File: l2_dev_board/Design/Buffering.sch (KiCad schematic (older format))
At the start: 32 parts, among them U202 NC7WZ07, U203 NC7WZ07, U204 NC7WZ07, U205 NC7WZ07, U302 NC7WZ17, U303 NC7WZ17, U304 NC7WZ17, U305 NC7WZ17, U306 NC7WZ17, U307 NC7WZ17, U310 NC7WZ17, U311 NC7WZ17

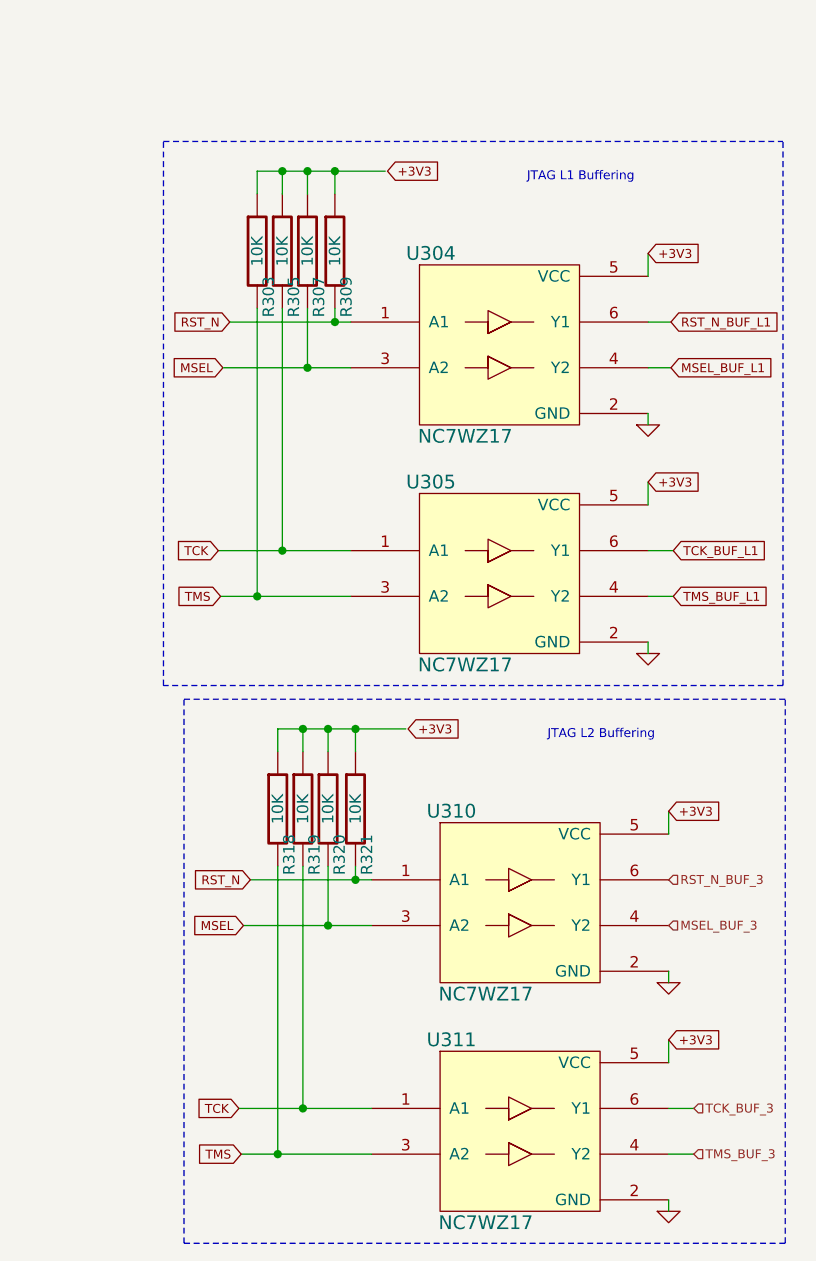
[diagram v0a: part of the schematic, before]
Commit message: missing header connector for 2 L2s. Find space!
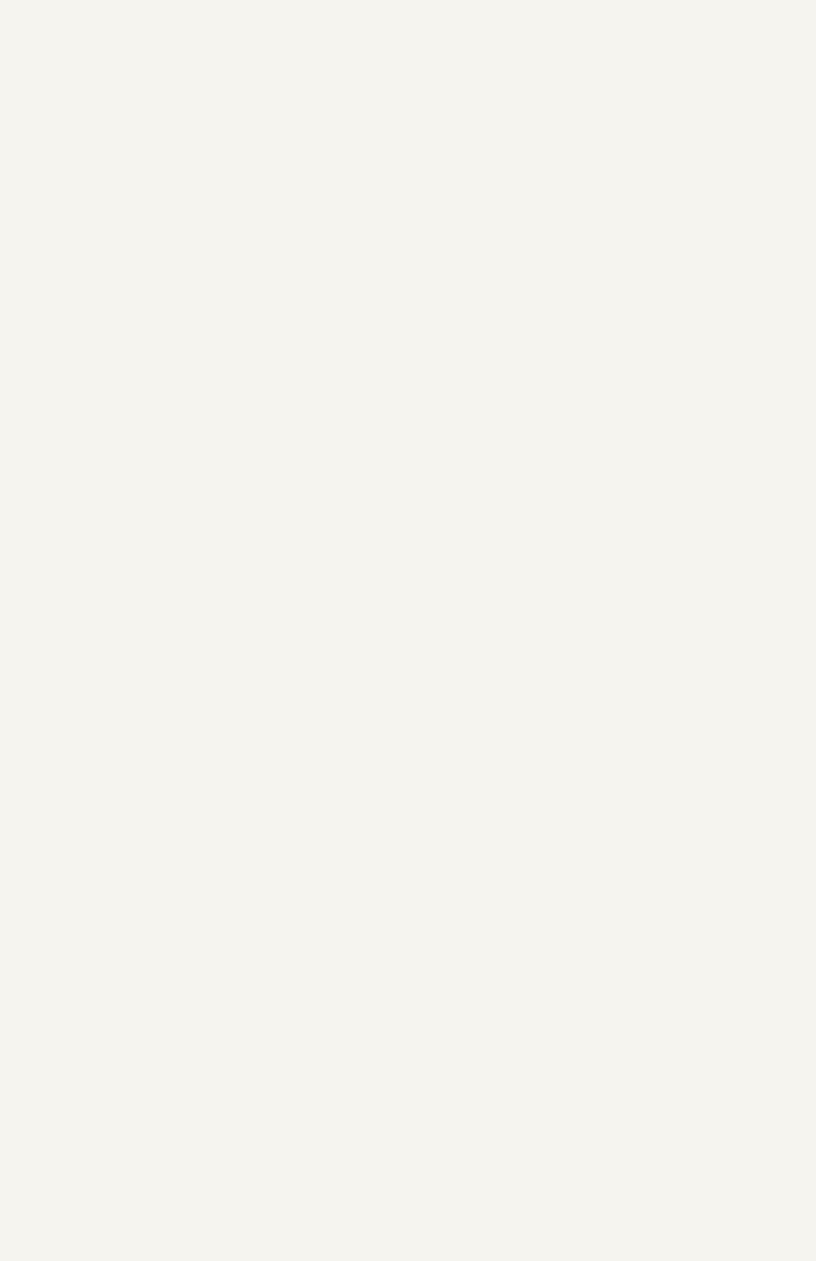
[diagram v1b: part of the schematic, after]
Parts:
- removed R303, R305, R307, R309, R318, R319, R320, R321: 10K, symbol R
- removed U304, U305, U310, U311: NC7WZ17, symbol NC7WZ17
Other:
- note removed: "JTAG L1 Buffering"
- note removed: "JTAG L2 Buffering"
